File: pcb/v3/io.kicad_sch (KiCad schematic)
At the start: 66 parts, among them J12 Conn_01x04, J13 Conn_01x05, P1 LCD_MIPI, P2 LCD_TOUCH, Q3 NMOS, U10 STI9287, U11 TXS0102DCU, U13 TS3A227E, Y1 24.576M

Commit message: pcb 3.9
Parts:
- U11: footprint Package_SO:VSSOP-8_2.3x2mm_P0.5mm -> Package_SON:X2SON-8_1.4x1mm_P0.35mm
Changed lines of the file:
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@@
 			)
 		)
-		(property "Footprint" "Package_SO:VSSOP-8_2.3x2mm_P0.5mm"
+		(property "Footprint" "Package_SON:X2SON-8_1.4x1mm_P0.35mm"
 			(at 171.45 140.97 0)
 			(effects

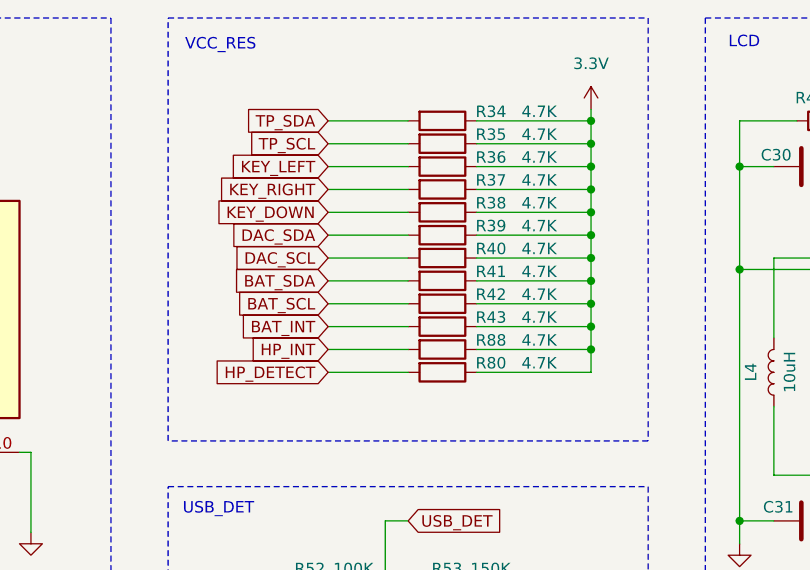
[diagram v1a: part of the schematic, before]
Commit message: pcb
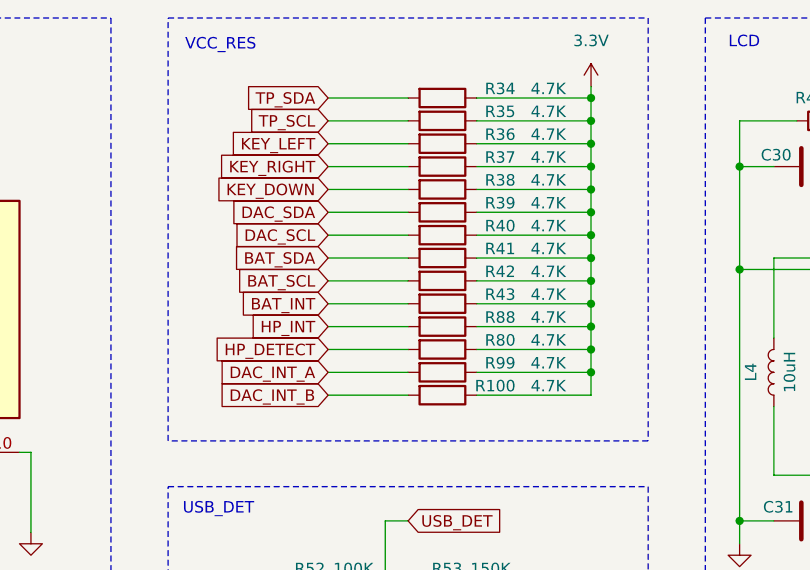
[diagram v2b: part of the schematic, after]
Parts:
- added R100, R99: 4.7K, Capacitor_SMD:C_0402_1005Metric_Pad0.74x0.62mm_HandSolder, symbol Device:R
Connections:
- net 3.3V: now also R100.1, R99.1
- new net DAC_INT_A: R99.2
- new net DAC_INT_B: R100.2
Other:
- moved on the sheet: R34, R35, R36, R37, R38, R39, R40, R41, R42, R43, R80, R88

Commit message: 3.11
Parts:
- U11: footprint Package_SON:X2SON-8_1.4x1mm_P0.35mm -> Package_SO:VSSOP-8_2.3x2mm_P0.5mm
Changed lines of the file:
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@@
 			)
 		)
-		(property "Footprint" "Package_SON:X2SON-8_1.4x1mm_P0.35mm"
+		(property "Footprint" "Package_SO:VSSOP-8_2.3x2mm_P0.5mm"
 			(at 171.45 140.97 0)
 			(effects
